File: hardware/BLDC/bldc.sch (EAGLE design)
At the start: 37 parts, among them J1 PWR_2_XT30PW-M, U1 MA702, U2 DRV8323RS, U3 TPN7R006PL, U4 TPN7R006PL, U5 TPN7R006PL, U6 TPN7R006PL, U7 TPN7R006PL, U8 TPN7R006PL, U9 STM32G4_UFQFPN48_T1

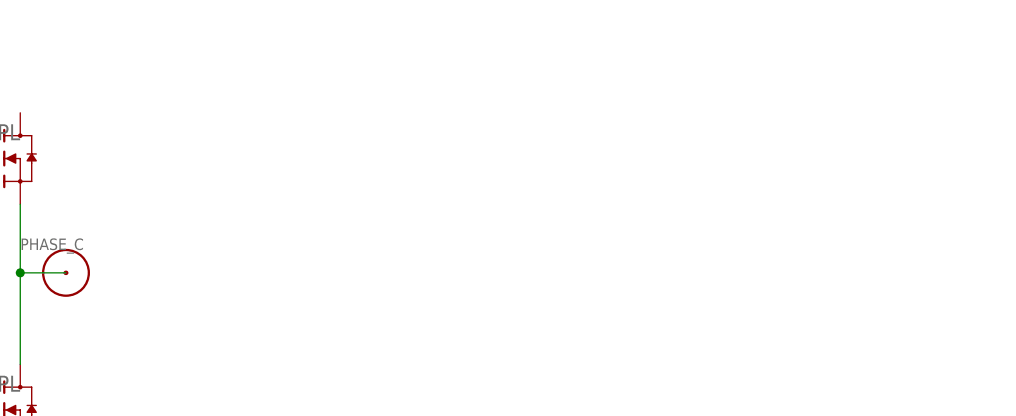
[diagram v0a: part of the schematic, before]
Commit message: Added bulk caps
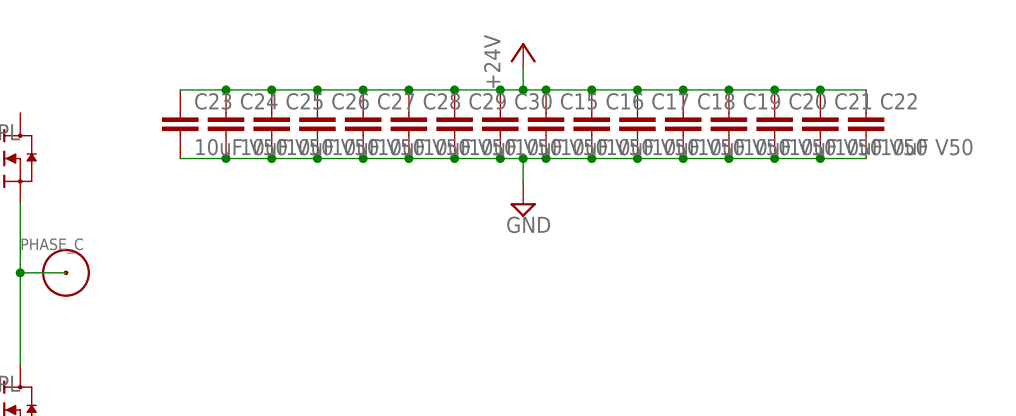
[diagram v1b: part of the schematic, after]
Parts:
- added C15, C16, C17, C18, C19, C20, C21, C22, C23, C24, C25, C26, C27, C28, C29, C30: 10uF V50, _T_rcl:C1206
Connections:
- net +24V: now also C15.1, C16.1, C17.1, C18.1, C19.1, C20.1, C21.1, C22.1, C23.1, C24.1, C25.1, C26.1, C27.1, C28.1, C29.1, C30.1
- net GND: now also C15.2, C16.2, C17.2, C18.2, C19.2, C20.2, C21.2, C22.2, C23.2, C24.2, C25.2, C26.2, C27.2, C28.2, C29.2, C30.2
